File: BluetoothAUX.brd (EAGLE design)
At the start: 38.7 x 28.6 mm, 17 parts, among them IC2 TPA6132A2, X1 STEREOJACK, X2 MINI-USB-SCHIELD-32005-201

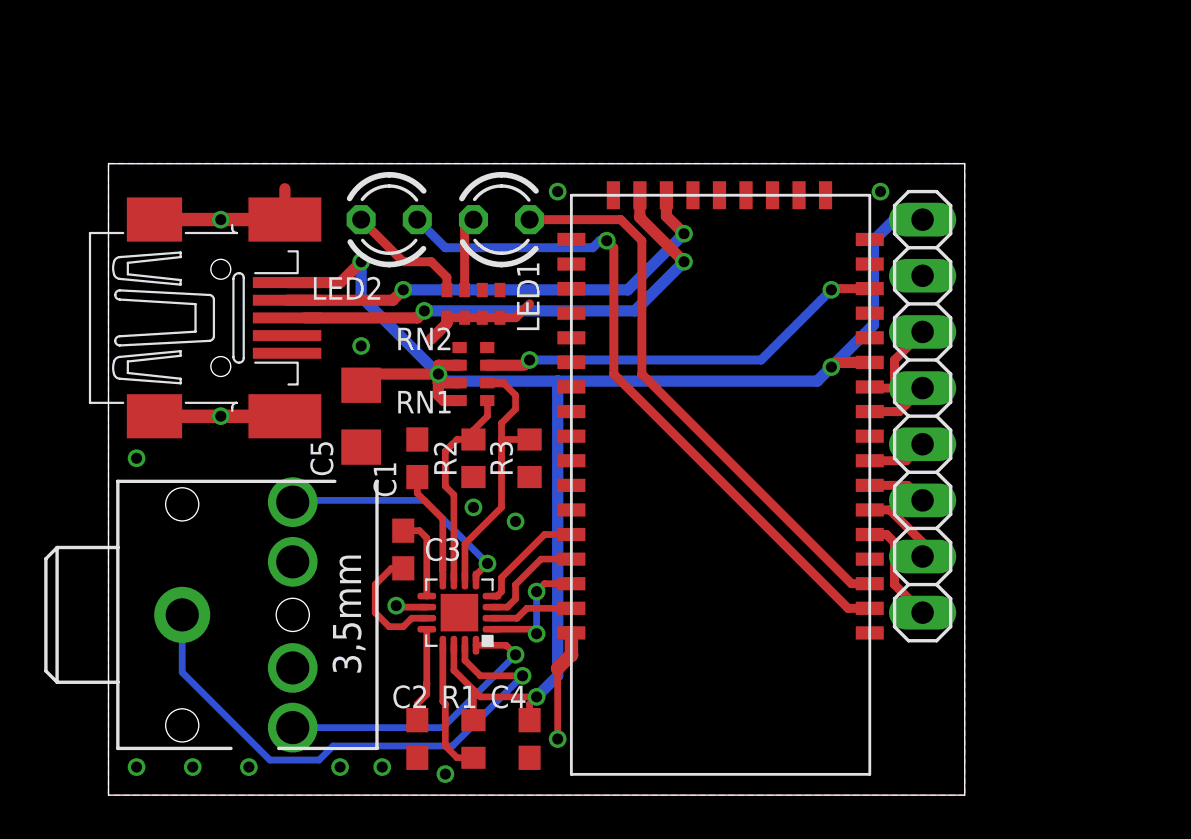
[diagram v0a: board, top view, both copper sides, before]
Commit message: Make smaller
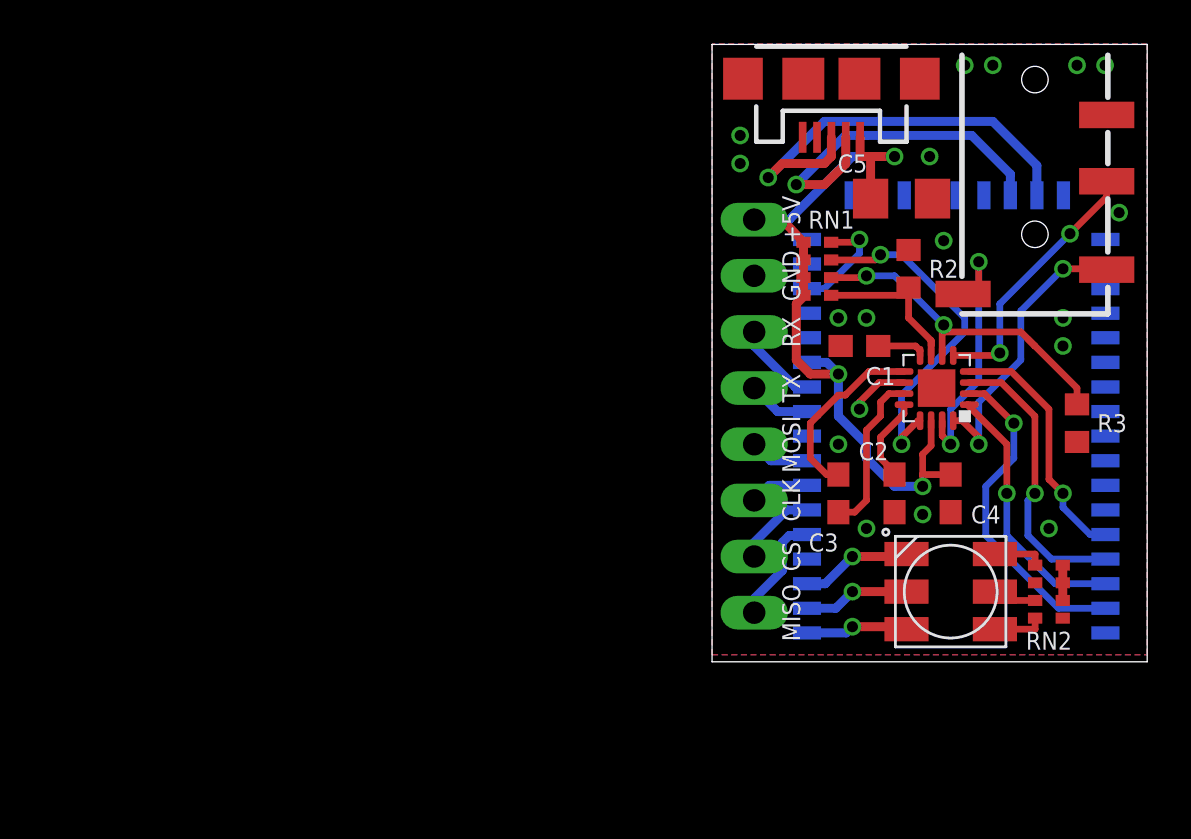
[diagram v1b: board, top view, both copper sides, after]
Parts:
- removed LED2: (no value), led:LED3MM
- removed R1: 10K, resistor:R0603
- removed X1: STEREOJACK, adafruit:STX3100
- removed X2: MINI-USB-SCHIELD-32005-201, con-cypressindustries:32005-201
- added J3: AUDIO_JACK_TRRSSMD_RA, SparkFun-Connectors:AUDIO_JACK_3.5MM_TRRS_SMD_RA
- added J4: USB, SparkFun-Connectors:USB-MICROB
- LED1: value (none) -> RGBLED5050; device led:LED3MM -> adafruit:RGBLED5050
- R2, R3: value (none) -> 0
- RN2: value 1K -> 220
- U$1: device BT:F3188 -> BluetoothAUX:F3188
- moved RN2 29.1 mm to (88.3, 24.4), turned to 90 degrees
- moved LED1 26.4 mm to (83.8, 24.4), turned to 180 degrees
- moved C5 26.4 mm to (81.6, 42.2), turned to 0 degrees
- moved R3 24.8 mm to (89.5, 32.1)
- moved C2 24.3 mm to (81.3, 28.9)
- moved IC2 23.9 mm to (83.2, 33.7)
- moved C4 22.1 mm to (83.8, 28.9)
- moved R2 21.5 mm to (81.9, 39.1), turned to 270 degrees
- moved C1 20.6 mm to (79.7, 35.6), turned to 180 degrees
- moved C3 19.8 mm to (78.7, 28.9)
- moved RN1 16.3 mm to (77.8, 39.1)
- moved U$1 10.2 mm to (83.8, 30.5), flipped to the bottom
- moved JP10 7.62 mm to (74.9, 32.4), flipped to the bottom
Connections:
- net N$26 renamed CPP
- net N$27 renamed CPN
- net N$28 renamed HPVSS
- net N$29 renamed HVPDD
- net N$31 renamed G0
- net N$32 renamed G1
- removed net LED1+: LED1.K, U$1.P$3
- removed net LED1-: LED1.A, RN2.7
- removed net LED2+: LED2.K, U$1.P$2
- removed net LED2-: LED2.A, RN2.8
- removed net N$13: RN1.3, U$1.P$15
- removed net N$14: IC2.5, X1.2
- removed net N$18: U$1.P$24, X2.2
- removed net N$19: U$1.P$25, X2.3
- removed net N$20: IC2.16, X1.5
- removed net N$30: IC2.13, R1.1
- new net LED0: LED1.4, U$1.P$3
- new net LED1: LED1.5, U$1.P$2
- new net LED2: LED1.6, U$1.P$1
- new net LED_B: LED1.3, RN2.5
- new net LED_G: LED1.1, RN2.8
- new net LED_R: LED1.2, RN2.7
- new net OUTL: IC2.16, J3.TIP
- new net OUTR: IC2.5, J3.RING1
- new net POWER_EN: RN1.4, U$1.P$15
- new net TPA_EN: IC2.13, RN1.3
- new net USB_N: J4.D-, U$1.P$24
- new net USB_P: J4.D+, U$1.P$25
- net +5V: now also J4.VBUS, RN1.5; no longer R1.2, X2.1
- net GND: now also J4.GND, J4.MT1, J4.MT2, J4.P$1, J4.P$2; no longer X2.5, X2.M1, X2.M2, X2.M3, X2.M4
- net SGND: now also J3.EARTH; no longer X1.1
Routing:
- net +5V: track 70.4 -> 36.0 mm, vias 4 -> 3
- net LED2+: track 31.4 -> 0.00 mm, vias 1 -> 0
- net LED1+: track 25.7 -> 0.00 mm
- net N$19: track 22.8 -> 0.00 mm, vias 2 -> 0
- net N$18: track 21.3 -> 0.00 mm, vias 2 -> 0
- net GND: track 25.2 -> 4.30 mm, vias 16 -> 18
- net USB_P: track 0.00 -> 19.5 mm, vias 0 -> 1
- net N$13: track 18.8 -> 0.00 mm, vias 2 -> 0
- net USB_N: track 0.00 -> 16.1 mm, vias 0 -> 1
- net TPA_EN: track 0.00 -> 15.7 mm, vias 0 -> 2
- net N$20: track 13.4 -> 0.00 mm, vias 1 -> 0
- net OUTL: track 0.00 -> 13.3 mm, vias 0 -> 2
- net SGND: track 24.8 -> 12.2 mm, vias 1 -> 2
- net OUTR: track 0.00 -> 11.9 mm, vias 0 -> 2
- net SPK_LP: track 3.78 -> 15.0 mm, vias 0 -> 1
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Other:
- board size 38.7 x 28.6 mm -> 19.7 x 27.9 mm
